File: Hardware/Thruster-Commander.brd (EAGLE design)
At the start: 50.8 x 20.3 mm, 27 parts, among them U5 MC7805, Y1 8Mhz

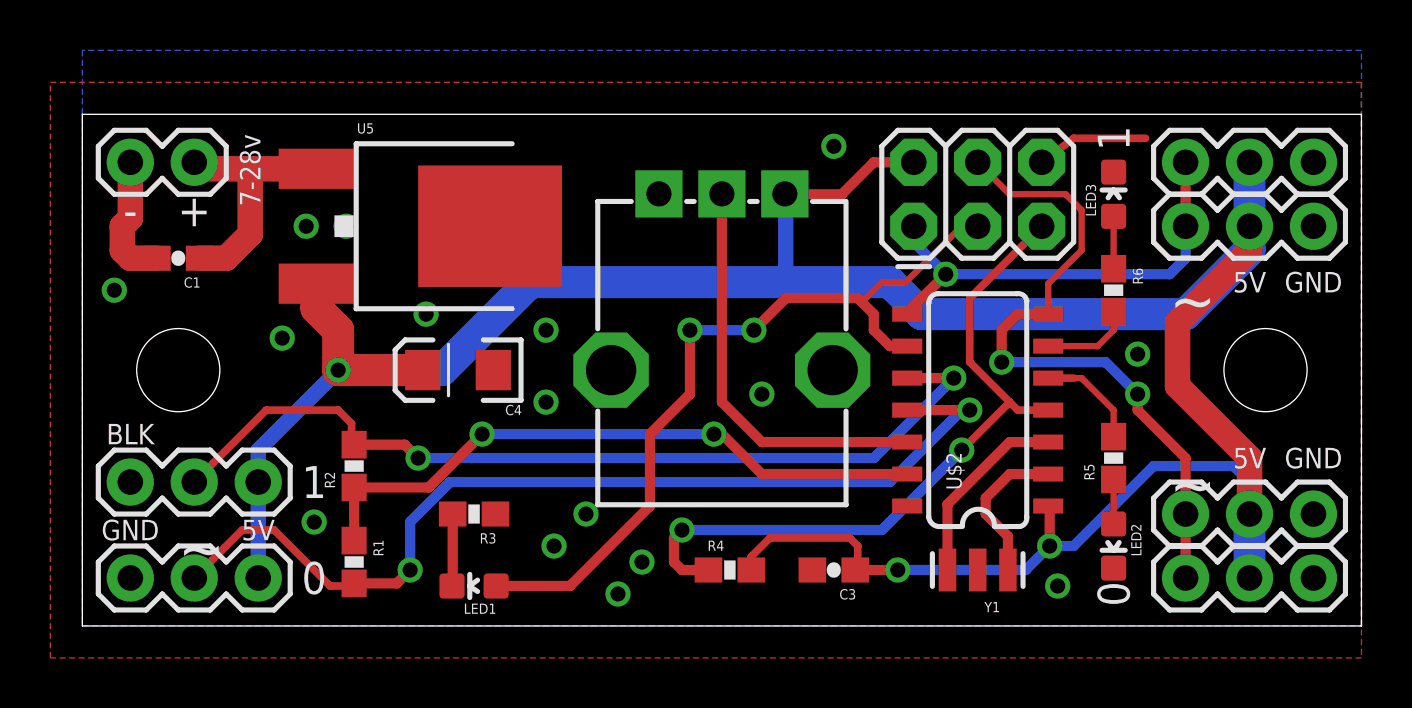
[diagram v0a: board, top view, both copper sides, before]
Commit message: Updates to rev4.
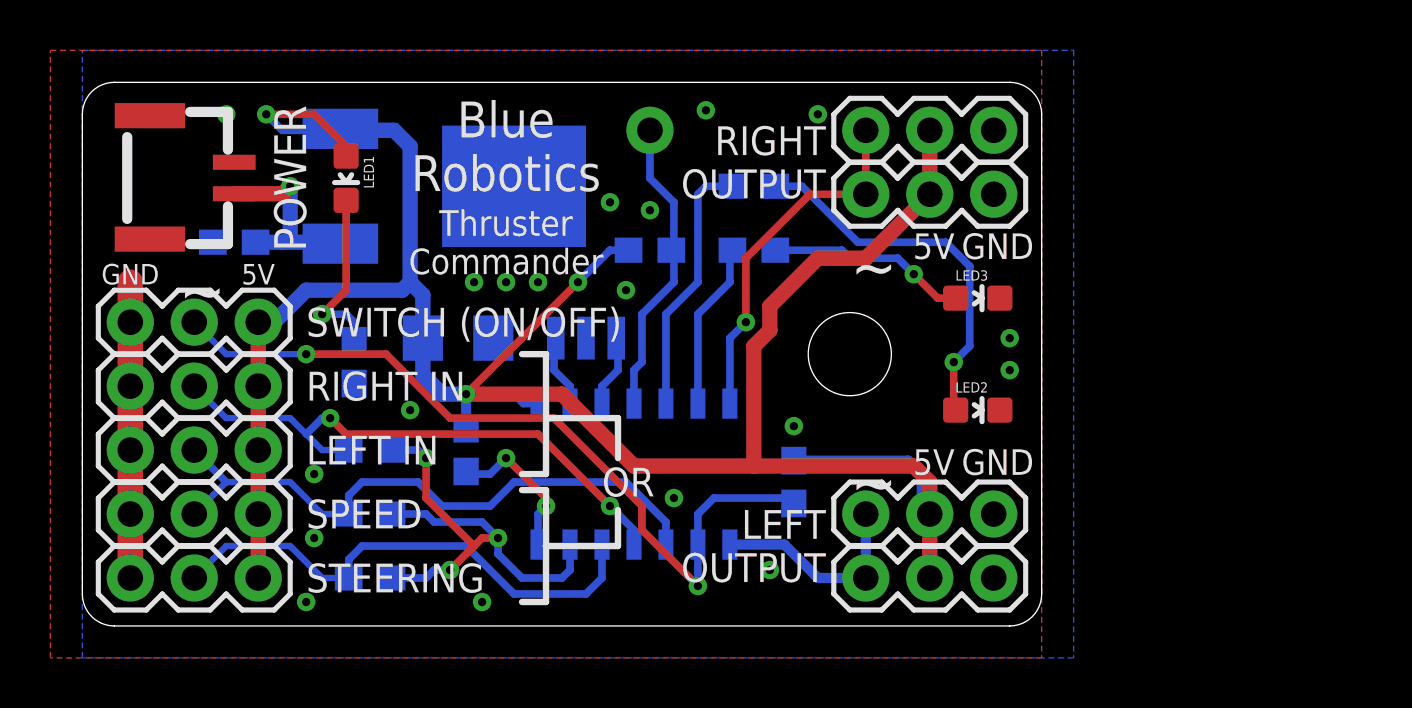
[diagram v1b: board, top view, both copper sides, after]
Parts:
- removed AVR_ICSP: (no value), SparkFun-Connectors:2X3
- removed C4: 22uF 10V, SparkFun-Capacitors:EIA3216
- removed IN_EXT1: (no value), SparkFun-Connectors:1X03
- removed JP1: (no value), SparkFun-Connectors:1X02
- removed POT1: (no value), SparkFun-Electromechanical:ALPS_POT
- removed STANDOFF2: STAND-OFF, SparkFun-Electromechanical:STAND-OFF
- added C2: 22uF 10V, SparkFun-Capacitors:1206
- added JP2: M01PTH, SparkFun-Connectors:1X01
- added R7: 10K, SparkFun-Resistors:0603-RES
- added R8: 100K, SparkFun-Resistors:0603-RES
- added SW, THR, THR0, THR1: (no value), SparkFun-Connectors:1X03
- added U$3: JSH-GH-2VERT, BlueRobotics-JST-GH:JST-GH-TOP-2
- R1, R2: value 1M -> 100K
- U$1: value LOGOFULL-M -> LOGOBR-LOGO-MS; device BlueRobotics-Main:BR-FULL-LOGO-MEDIUM -> BlueRobotics-Main:BR-LOGO-MEDIUM-SMALL
- moved STANDOFF1 26.7 mm to (30.5, 10.8)
- moved U$1 19.8 mm to (22.9, 6.35), flipped to the top
- moved Y1 18.1 mm to (20.0, 11.4), flipped to the bottom
- moved R5 17.9 mm to (26.7, 17.5), flipped to the bottom, turned to 0 degrees
- moved LED1 17.0 mm to (10.5, 17.8), turned to 180 degrees
- moved C3 15.4 mm to (15.2, 6.99), flipped to the bottom, turned to 270 degrees
- moved R6 14.4 mm to (26.7, 14.9), flipped to the bottom, turned to 0 degrees
- moved U$2 13.9 mm to (21.9, 6.03), flipped to the bottom, turned to 180 degrees
- moved R4 13.1 mm to (22.5, 14.9), flipped to the bottom
- moved PWM1A 12.8 mm to (31.1, 17.1)
- moved PWM1B 12.8 mm to (31.1, 19.7)
- moved PWM0A 12.7 mm to (31.1, 4.45)
- moved PWM0B 12.7 mm to (31.1, 1.91)
- moved R3 7.69 mm to (10.8, 10.5), flipped to the bottom, turned to 90 degrees
- moved LED2 7.63 mm to (35.6, 8.57), turned to 270 degrees
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- renumbered IN_EXT0 to STEER
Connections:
- removed net INPUT_EXT0: R1.2, STEER.2, U$2.11
- removed net INPUT_EXT1: IN_EXT1.2, R2.2, U$2.10
- removed net INPUT_INT: POT1.P$2, U$2.12
- removed net LED_INT: AVR_ICSP.3, LED1.A, U$2.9
- new net STEERING: R8.2, STEER.2, U$2.12
- new net SWITCH: R7.1, SW.2, U$2.9
- new net THROTTLE0: R1.2, THR0.2, U$2.11
- new net THROTTLE1: R2.2, THR.2, THR1.2, U$2.10
- net +5V: now also C2.1, LED1.A, R7.2, SW.3, THR.3, THR0.3, THR1.3; no longer AVR_ICSP.2, C4.A, IN_EXT1.3, POT1.P$1
- net DETECT: now also R8.1
- net GND: now also C2.2, SW.1, THR.1, THR0.1, THR1.1, U$3.2; no longer AVR_ICSP.6, C4.C, IN_EXT1.1, JP1.1, POT1.P$3
- net PWM0: now also U$2.8; no longer AVR_ICSP.4, U$2.7
- net PWM1: now also U$2.7; no longer AVR_ICSP.1, U$2.8
- net RESET: now also JP2.1; no longer AVR_ICSP.5
- net VIN: now also U$3.1; no longer JP1.2
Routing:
- net INPUT_EXT0: track 39.0 -> 0.00 mm, vias 2 -> 0
- net INPUT_EXT1: track 35.7 -> 0.00 mm, vias 2 -> 0
- net SWITCH: track 0.00 -> 31.9 mm, vias 0 -> 2
- net LED_INT: track 31.2 -> 0.00 mm, vias 2 -> 0
- net THROTTLE1: track 0.00 -> 24.9 mm
- net THROTTLE0: track 0.00 -> 22.9 mm, vias 0 -> 2
- net STEERING: track 0.00 -> 20.6 mm
- net PWM0: track 27.0 -> 8.49 mm, vias 2 -> 0
- net RESET: track 28.5 -> 12.0 mm, vias 2 -> 0
- net INPUT_INT: track 16.3 -> 0.00 mm
- net N$2: track 1.77 -> 15.0 mm, vias 0 -> 1
- net +5V: track 111.7 -> 99.8 mm
- net GND: track 9.57 -> 18.2 mm, vias 16 -> 21
- net LED_EXT0: track 4.18 -> 10.3 mm
- net N$5: track 2.08 -> 7.95 mm, vias 0 -> 1
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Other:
- board size 50.8 x 20.3 mm -> 38.1 x 21.6 mm
- board text added: "7-28V"
- board text added: "Blue Robotics"
- board text added: "LEFT IN"
- board text added: "LEFT OUTPUT"
- board text added: "OR"
- board text added: "POWER"
- board text added: "RESET"
- board text added: "RIGHT IN"
- board text added: "RIGHT OUTPUT"
- board text added: "SPEED"
- board text added: "STEERING"
- board text added: "SWITCH (ON/OFF)"
- board text added: "rev4 - 10/17"
- board text removed: "+"
- board text removed: "-"
- board text removed: "0"
- board text removed: "1"
- board text removed: "7-28v"
- board text removed: "BLK"
- board text removed: "IN 0"
- board text removed: "IN 1"
- board text removed: "PWM0"
- board text removed: "PWM1"
- board text removed: "PWR"
- board text removed: "rev3 - 10/17"
